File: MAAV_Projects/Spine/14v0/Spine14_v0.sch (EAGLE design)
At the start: 96 parts, among them IC3 PINTO_SMD, J7 MA04-1, Q3 MOSFET-NCHANNELBSS138, Q4 MOSFET-NCHANNELBSS138, Q5 32.768KHz, Q6 16MHz, Q7 CRYSTAL_16MHZ_SMD, Q8 MOSFET-NCHANNELBSS138, Q9 MOSFET-NCHANNELBSS138, U1 ATMEGA328-AU, U2 REG_3V_8SOIC

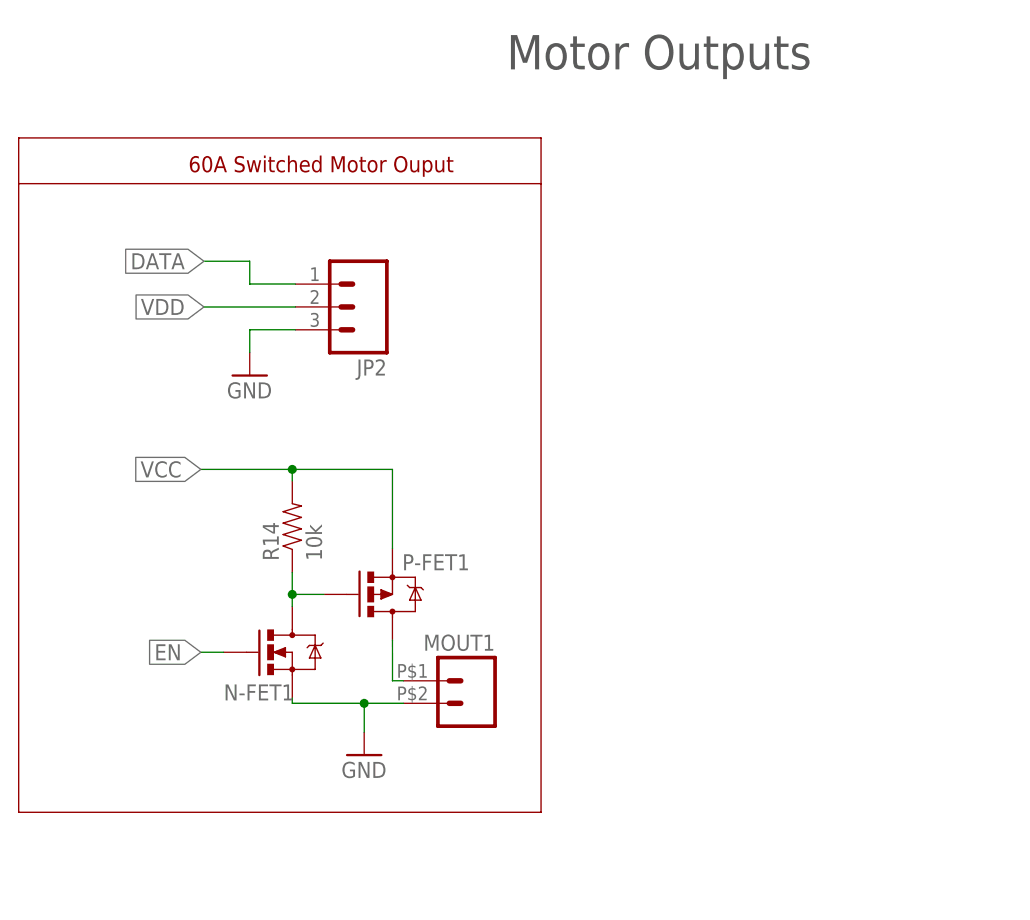
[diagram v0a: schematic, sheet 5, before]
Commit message: blah
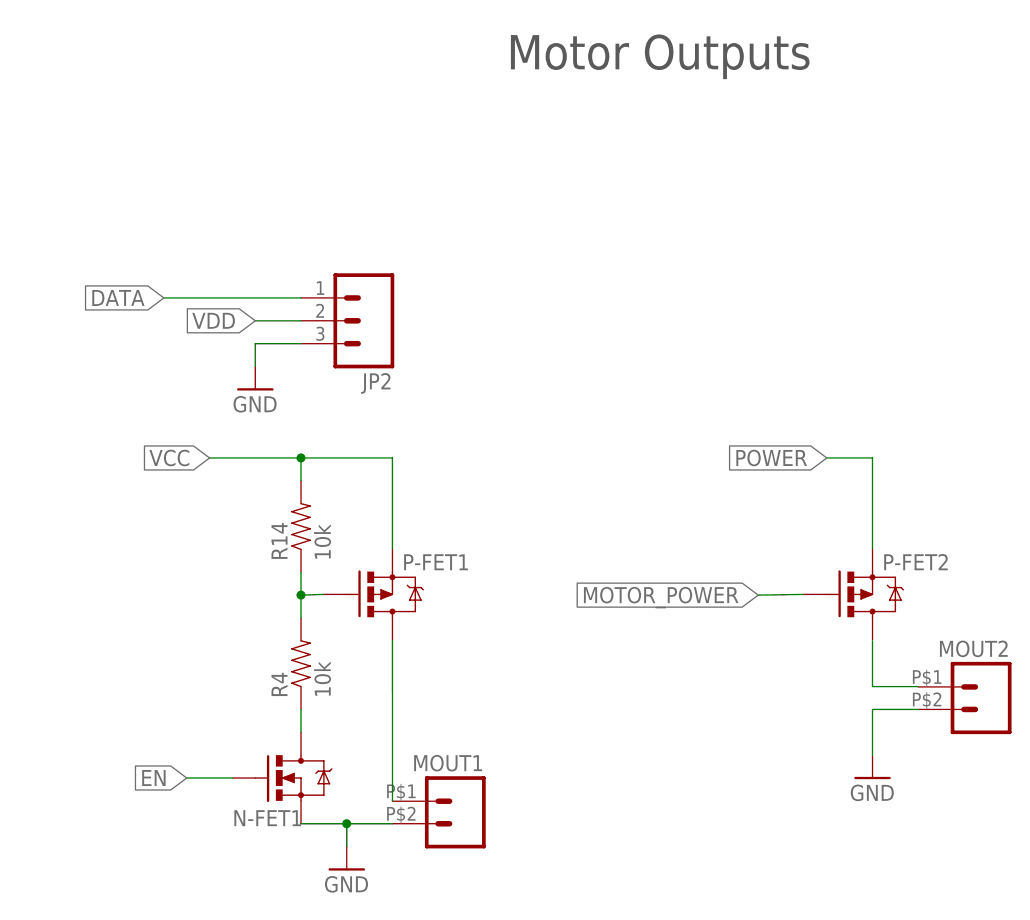
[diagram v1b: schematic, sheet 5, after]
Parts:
- added MOUT2: MINI_FIT_JR_5569, SAUVE:MINI_FIT_JR_5569
- added P-FET2: MOSFET_P-CHANNEL, SAUVE:MOSFET_P-CHANNEL
- added Q1: MOSFET-NCHANNELBSS138, SparkFun-DiscreteSemi:MOSFET-NCHANNELBSS138
- added R3: 10k, rcl:R-US_R0603
- added R4: 10k, SparkFun-Resistors:RESISTOR0603-RES
- R2: value 432 -> 10k
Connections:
- removed net N$17: MOUT1.1, N-FET1.S
- new net N$1: Q1.D, R2.1
- new net N$2: N-FET1.D, R4.1
- net GND: now also MOUT1.1, MOUT2.1, N-FET1.S, Q1.S, R3.1; no longer R2.1
- net MOTOR_LOGIC: now also Q1.G, R3.2
- net MOTOR_POWER: now also P-FET2.G
- net N$16: now also R4.2; no longer N-FET1.D
- net POWER: now also P-FET2.S
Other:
- note removed: "60A Switched Motor Ouput"
- moved on the sheet: I2C_1, I2C_2, JP2, MOUT1, N-FET1, R14, R2

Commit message: too tired. will finish motors later
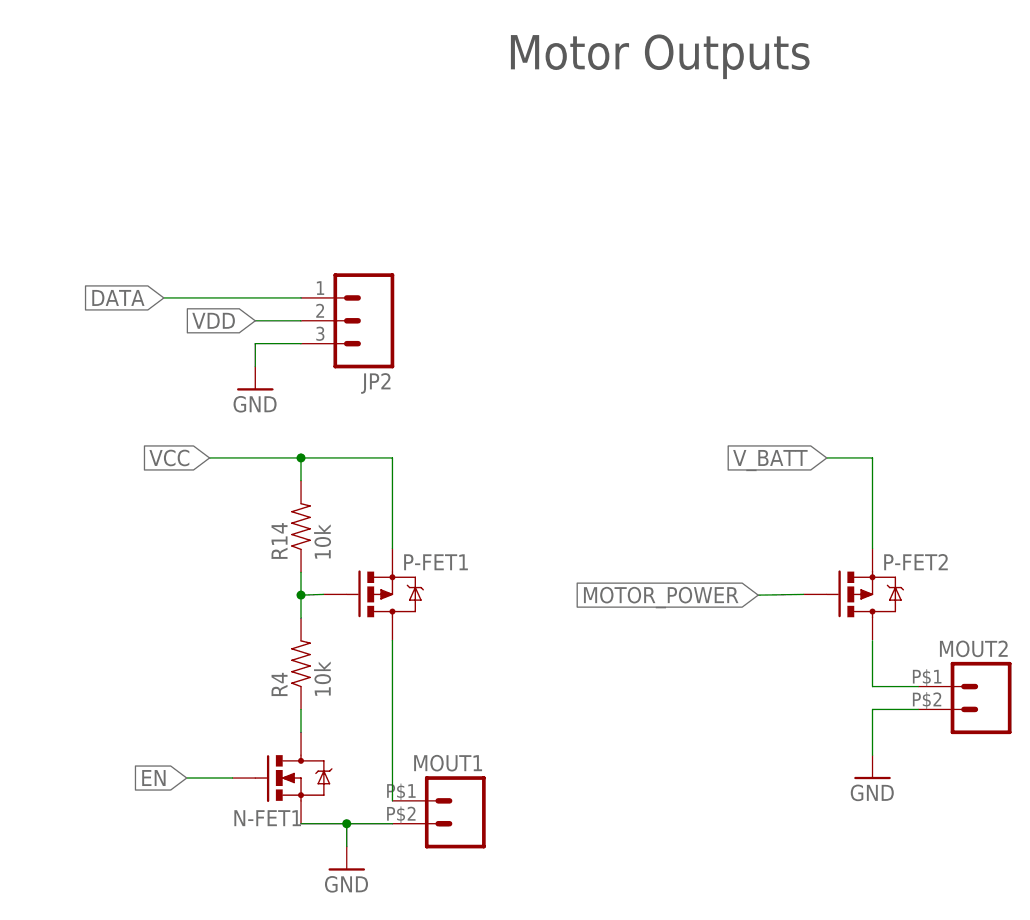
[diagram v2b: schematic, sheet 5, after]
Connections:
- new net N$3: MOUT2.2
- net POWER: no longer P-FET2.S
- net V_BATT: now also P-FET2.S
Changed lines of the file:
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@@
 <segment>
 <wire x1="-30.48" y1="-20.24" x2="-30.477459375" y2="-37.46" width="0.1524" layer="91"/>
-<wire x1="-30.477459375" y1="-37.46" x2="-30.48" y2="-38.14" width="0.1524" layer="91"/>
+<wire x1="-30.477459375" y1="-37.46" x2="-30.48" y2="-38.1" width="0.1524" layer="91"/>
 <pinref part="P-FET1" gate="G$1" pin="D"/>
 <pinref part="MOUT1" gate="G$1" pin="2"/>
@@
 </segment>
 </net>
-<net name="POWER" class="0">
+<net name="N$3" class="0">
+<segment>
+<wire x1="22.86" y1="-25.4" x2="22.86" y2="-20.32" width="0.1524" layer="91"/>
+<pinref part="MOUT2" gate="G$1" pin="2"/>
+<wire x1="22.86" y1="-25.4" x2="27.94" y2="-25.4" width="0.1524" layer="91"/>
+</segment>
+</net>
+<net name="V_BATT" class="0">
 <segment>
 <label x="17.78" y="0" size="1.778" layer="95" rot="R180" xref="yes"/>
@@
 </segment>
 </net>
-<net name="N$3" class="0">
-<segment>
-<wire x1="27.94" y1="-25.4" x2="22.86" y2="-25.4" width="0.1524" layer="91"/>
-<wire x1="22.86" y1="-25.4" x2="22.86" y2="-20.32" width="0.1524" layer="91"/>
-</segment>
-</net>
